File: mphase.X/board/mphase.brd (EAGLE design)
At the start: 120.6 x 82.2 mm, 36 parts, among them IC1 MAX232, IC2 PIC18F4455_40, X1 332-10, X2 332-10

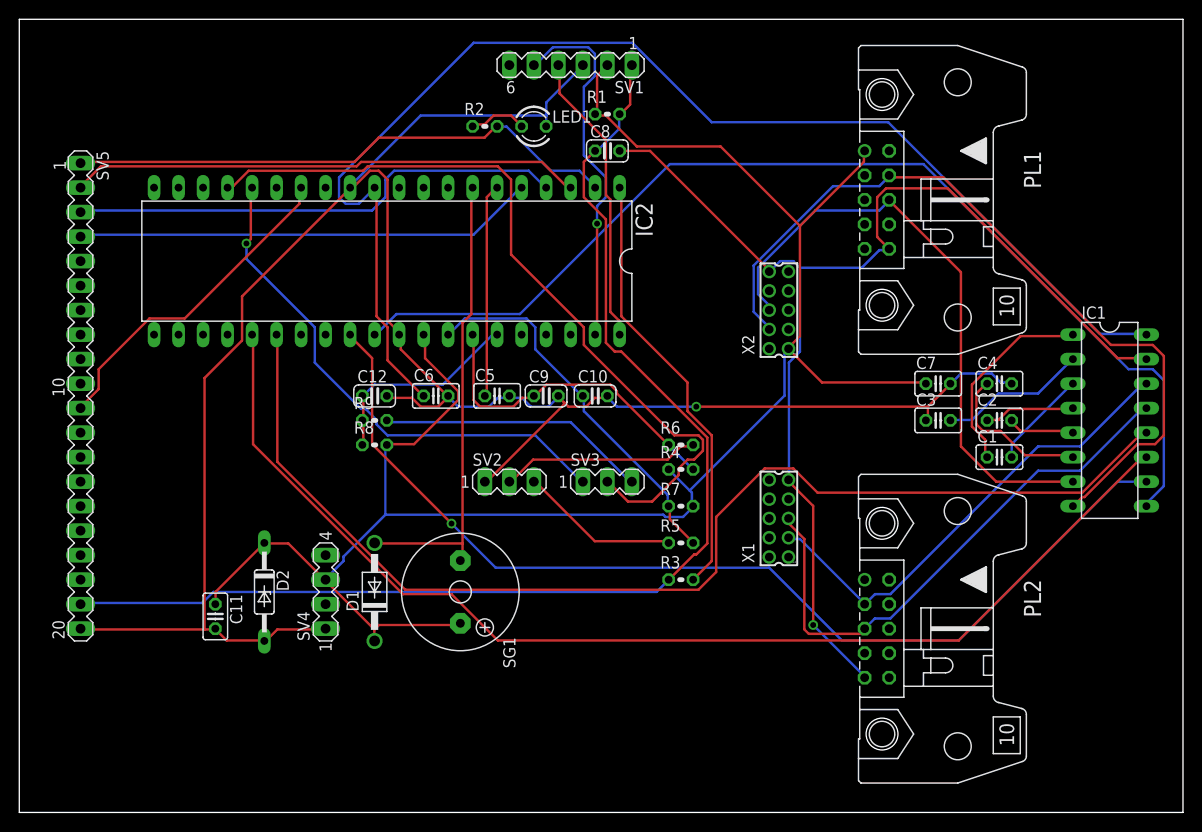
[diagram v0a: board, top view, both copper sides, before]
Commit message: up
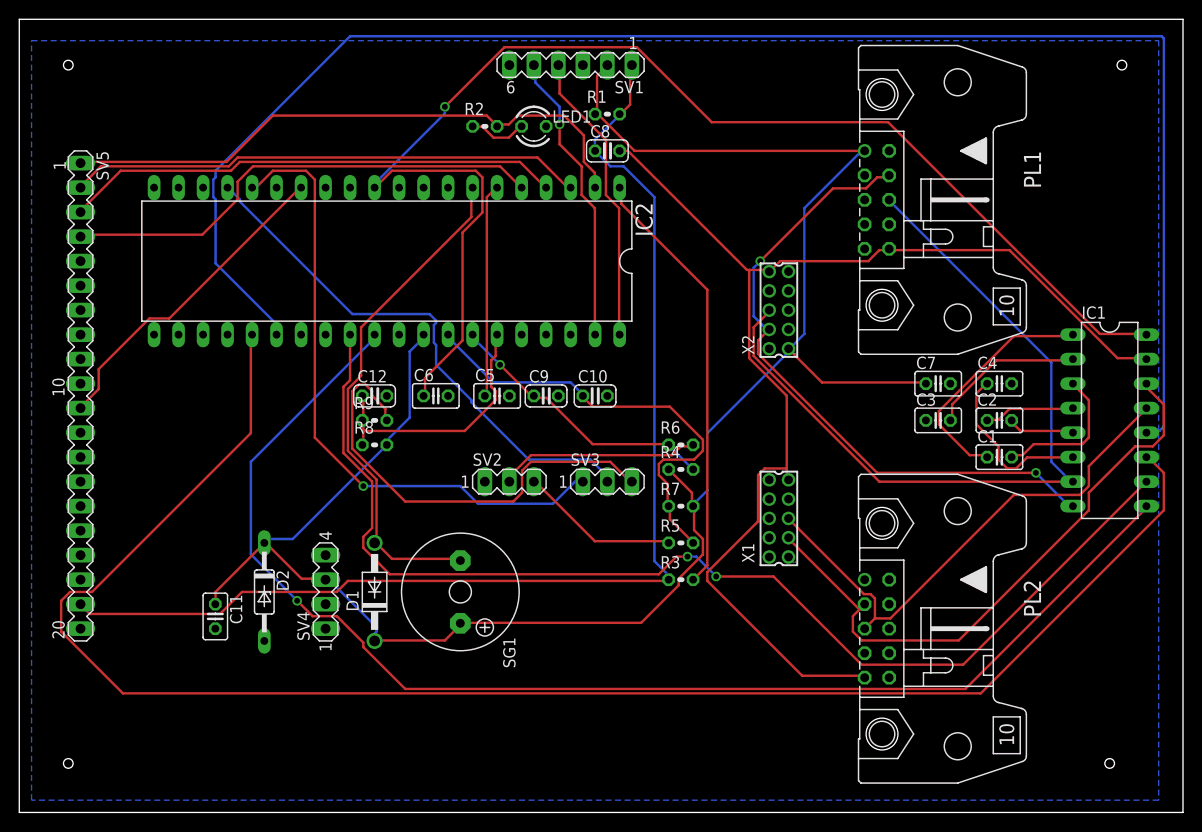
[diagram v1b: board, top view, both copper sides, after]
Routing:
- net VSS: track 224.9 -> 0.00 mm, vias 1 -> 0
- net N$11: track 120.3 -> 171.5 mm
- net N$12: track 121.0 -> 166.3 mm
- net N$34: track 82.0 -> 55.5 mm
- net N$13: track 112.3 -> 134.9 mm, vias 0 -> 1
- net N$31: track 28.1 -> 47.4 mm
- net N$16: track 63.1 -> 81.1 mm
- net N$17: track 82.2 -> 67.6 mm, vias 0 -> 2
- net N$19: track 49.5 -> 62.5 mm
- net N$10: track 107.8 -> 119.6 mm, vias 1 -> 2
- net N$33: track 54.5 -> 65.9 mm
- net N$22: track 39.3 -> 47.3 mm
- net N$32: track 38.4 -> 30.6 mm
- net N$28: track 21.8 -> 27.5 mm
- net N$21: track 34.6 -> 29.0 mm, vias 0 -> 1
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- added copper zone on layer 16, net VSS
